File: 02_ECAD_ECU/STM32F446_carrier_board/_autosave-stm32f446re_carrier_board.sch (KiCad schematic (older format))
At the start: 30 parts, among them SW1 SW_SPDT, U1 STM32F446RETx, Y1 16MHz, Y2 32.768kHz

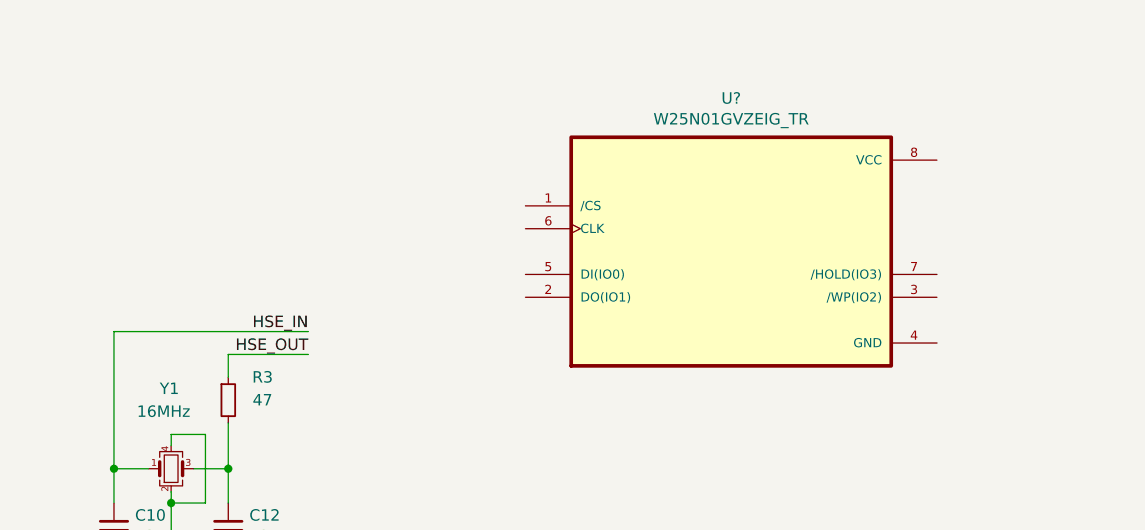
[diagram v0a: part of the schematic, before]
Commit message: carrierboard stm32f446 finished v0.1
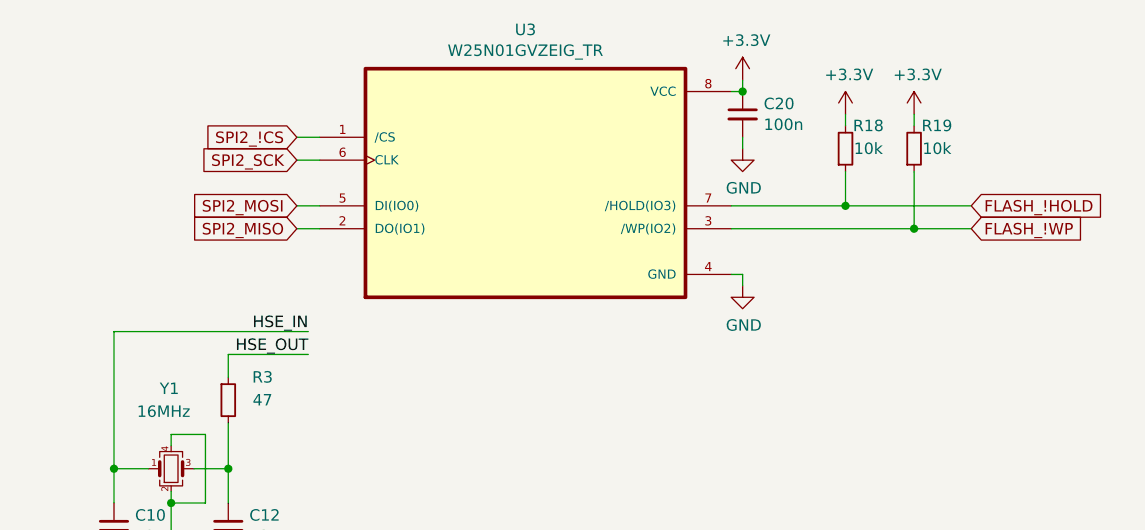
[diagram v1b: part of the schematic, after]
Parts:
- added C20: 100n, Capacitor_SMD:C_0603_1608Metric, symbol Device:C_Small
- added R18, R19: 10k, Resistor_SMD:R_1206_3216Metric, symbol Device:R_Small
- U3: renamed from U?; LCSC part # (none) -> C88868
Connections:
- net +3V3: now also U3.8 (VCC), C20.1, R18.2, R19.2
- net FLASH_!HOLD: now also U3.7 (/HOLD(IO3)), R18.1
- net FLASH_!WP: now also U3.3 (/WP(IO2)), R19.1
- net GND: now also U3.4 (GND), C20.2
- net SPI2_!CS: now also U3.1 (/CS)
- net SPI2_MISO: now also U3.2 (DO(IO1))
- net SPI2_MOSI: now also U3.5 (DI(IO0))
- net SPI2_SCK: now also U3.6 (CLK)
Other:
- moved on the sheet: U3
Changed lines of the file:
@@
 PB10
 $Comp
-L max_KiCAD_lib:W25N01GVZEIG_TR U?
+L max_KiCAD_lib:W25N01GVZEIG_TR U3
 U 1 1 61480725
-P 9350 1750
-F 0 "U?" H 9350 2420 50  0000 C CNN
-F 1 "W25N01GVZEIG_TR" H 9350 2329 50  0000 C CNN
-F 2 "max_KiCAD_lib:SON127P800X600X80-9N" H 9350 1750 50  0001 L BNN
-F 3 "" H 9350 1750 50  0001 L BNN
-F 4 "None" H 9350 1750 50  0001 L BNN "PRICE"
-F 5 "IPC7351B" H 9350 1750 50  0001 L BNN "STANDARD"
-F 6 "WSON-8 Winbond" H 9350 1750 50  0001 L BNN "PACKAGE"
-F 7 "Winbond Electronics" H 9350 1750 50  0001 L BNN "MANUFACTURER"
-F 8 "Ic Flash 1gbit 104mhz 8wson" H 9350 1750 50  0001 L BNN "DESCRIPTION"
-F 9 "W25N01GVZEIG TR" H 9350 1750 50  0001 L BNN "MP"
-	1    9350 1750
+P 8450 1450
+F 0 "U3" H 8450 2120 50  0000 C CNN
+F 1 "W25N01GVZEIG_TR" H 8450 2029 50  0000 C CNN
+F 2 "max_KiCAD_lib:SON127P800X600X80-9N" H 8450 1450 50  0001 L BNN
+F 3 "" H 8450 1450 50  0001 L BNN
+F 4 "None" H 8450 1450 50  0001 L BNN "PRICE"
+F 5 "IPC7351B" H 8450 1450 50  0001 L BNN "STANDARD"
+F 6 "WSON-8 Winbond" H 8450 1450 50  0001 L BNN "PACKAGE"
+F 7 "Winbond Electronics" H 8450 1450 50  0001 L BNN "MANUFACTURER"
+F 8 "Ic Flash 1gbit 104mhz 8wson" H 8450 1450 50  0001 L BNN "DESCRIPTION"
+F 9 "W25N01GVZEIG TR" H 8450 1450 50  0001 L BNN "MP"
+F 10 "C88868" H 8450 1450 50  0001 C CNN "LCSC part #"
+	1    8450 1450
 	1    0    0    -1
 $EndComp
+Text GLabel 7450 1250 0    50   Input ~ 0
+SPI2_!CS
+Text GLabel 7450 1350 0    50   Input ~ 0
+SPI2_SCK
+Text GLabel 7450 1650 0    50   Input ~ 0
+SPI2_MISO
+Text GLabel 7450 1550 0    50   Input ~ 0
+SPI2_MOSI
+Wire Wire Line
+	7450 1650 7550 1650
+Wire Wire Line
+	7450 1250 7550 1250
+Wire Wire Line
+	7450 1350 7550 1350
+Wire Wire Line
+	7450 1550 7550 1550
+$Comp
+L power:GND #PWR0138
+U 1 1 614C487E
+P 9400 1900
+F 0 "#PWR0138" H 9400 1650 50  0001 C CNN
+F 1 "GND" H 9405 1727 50  0000 C CNN
+F 2 "" H 9400 1900 50  0001 C CNN
+F 3 "" H 9400 1900 50  0001 C CNN
+	1    9400 1900
+	1    0    0    -1
+$EndComp
+Wire Wire Line
+	9350 1850 9400 1850
+Wire Wire Line
+	9400 1850 9400 1900
+$Comp
+L power:+3.3V #PWR0139
+U 1 1 614CDE88
+P 9400 1000
+F 0 "#PWR0139" H 9400 850 50  0001 C CNN
+F 1 "+3.3V" H 9415 1173 50  0000 C CNN
+F 2 "" H 9400 1000 50  0001 C CNN
+F 3 "" H 9400 1000 50  0001 C CNN
+	1    9400 1000
+	1    0    0    -1
+$EndComp
+Wire Wire Line
+	9350 1050 9400 1050
+Wire Wire Line
+	9400 1050 9400 1000
+$Comp
+L Device:C_Small C20
+U 1 1 614D74C0
+P 9400 1150
+F 0 "C20" H 9492 1196 50  0000 L CNN
+F 1 "100n" H 9492 1105 50  0000 L CNN
+F 2 "Capacitor_SMD:C_0603_1608Metric" H 9400 1150 50  0001 C CNN
+F 3 "~" H 9400 1150 50  0001 C CNN
+F 4 "C14663" H 9400 1150 50  0001 C CNN "LCSC part #"
+	1    9400 1150
+	1    0    0    -1
+$EndComp
+Connection ~ 9400 1050
+$Comp
+L power:GND #PWR0140
+U 1 1 614D7DB2
+P 9400 1300
+F 0 "#PWR0140" H 9400 1050 50  0001 C CNN
+F 1 "GND" H 9405 1127 50  0000 C CNN
+F 2 "" H 9400 1300 50  0001 C CNN
+F 3 "" H 9400 1300 50  0001 C CNN
+	1    9400 1300
+	1    0    0    -1
+$EndComp
+Wire Wire Line
+	9400 1250 9400 1300
+Text GLabel 10400 1550 2    50   Input ~ 0
+FLASH_!HOLD
+Text GLabel 10400 1650 2    50   Input ~ 0
+FLASH_!WP
+Wire Wire Line
+	9350 1550 9850 1550
+Wire Wire Line
+	10400 1650 10150 1650
+$Comp
+L power:+3.3V #PWR0141
+U 1 1 61530514
+P 9850 1150
+F 0 "#PWR0141" H 9850 1000 50  0001 C CNN
+F 1 "+3.3V" H 9865 1323 50  0000 C CNN
+F 2 "" H 9850 1150 50  0001 C CNN
+F 3 "" H 9850 1150 50  0001 C CNN
+	1    9850 1150
+	1    0    0    -1
+$EndComp
+$Comp
+L power:+3.3V #PWR0142
+U 1 1 615309F9
+P 10150 1150
+F 0 "#PWR0142" H 10150 1000 50  0001 C CNN
+F 1 "+3.3V" H 10165 1323 50  0000 C CNN
+F 2 "" H 10150 1150 50  0001 C CNN
+F 3 "" H 10150 1150 50  0001 C CNN
+	1    10150 1150
+	1    0    0    -1
+$EndComp
+$Comp
+L Device:R_Small R18
+U 1 1 61530C68
+P 9850 1300
+F 0 "R18" H 9950 1200 50  0000 C CNN
+F 1 "10k" H 9950 1300 50  0000 C CNN
+F 2 "Resistor_SMD:R_1206_3216Metric" H 9850 1300 50  0001 C CNN
+F 3 "~" H 9850 1300 50  0001 C CNN
+F 4 "C17902" H 9850 1300 50  0001 C CNN "LCSC part #"
+	1    9850 1300
+	1    0    0    1
+$EndComp
+Wire Wire Line
+	9850 1150 9850 1200
+Wire Wire Line
+	9850 1400 9850 1550
+Connection ~ 9850 1550
+Wire Wire Line
+	9850 1550 10400 1550
+$Comp
+L Device:R_Small R19
+U 1 1 6154C7CE
+P 10150 1300
+F 0 "R19" H 10250 1200 50  0000 C CNN
+F 1 "10k" H 10250 1300 50  0000 C CNN
+F 2 "Resistor_SMD:R_1206_3216Metric" H 10150 1300 50  0001 C CNN
+F 3 "~" H 10150 1300 50  0001 C CNN
+F 4 "C17902" H 10150 1300 50  0001 C CNN "LCSC part #"
+	1    10150 1300
+	1    0    0    1
+$EndComp
+Wire Wire Line
+	10150 1150 10150 1200
+Wire Wire Line
+	10150 1400 10150 1650
+Connection ~ 10150 1650
+Wire Wire Line
+	10150 1650 9350 1650
 $EndSCHEMATC
